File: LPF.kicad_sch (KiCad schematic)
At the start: 7 parts

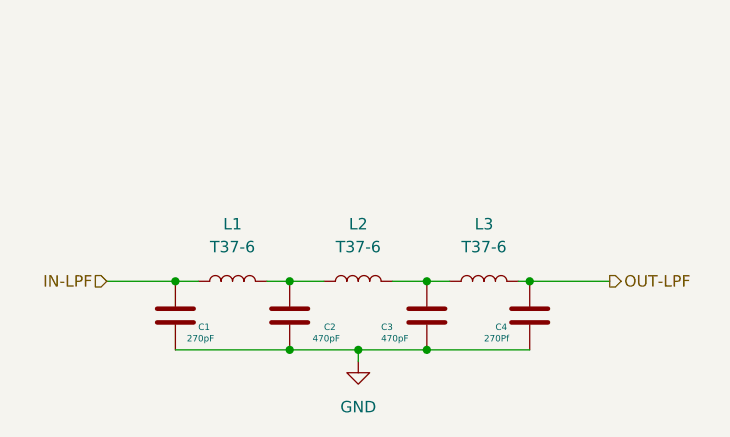
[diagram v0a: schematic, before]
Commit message: gg
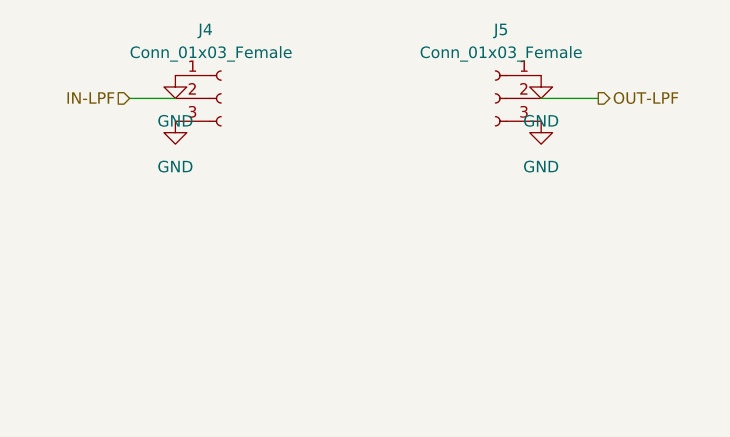
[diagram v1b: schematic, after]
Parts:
- removed C1: 270pF, Capacitor_SMD:C_1206_3216Metric, symbol Xenir:Capacitor
- removed C2, C3: 470pF, Capacitor_SMD:C_1206_3216Metric, symbol Xenir:Capacitor
- removed C4: 270Pf, Capacitor_SMD:C_1206_3216Metric, symbol Xenir:Capacitor
- removed L1, L2, L3: T37-6, Xenir:T37_Inductor, symbol Xenir:Inductor
- added J4, J5: Conn_01x03_Female, Connector_PinSocket_2.54mm:PinSocket_1x03_P2.54mm_Vertical, symbol Connector:Conn_01x03_Female
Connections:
- net GND: now also J4.1 (Pin_1), J4.3 (Pin_3), J5.1 (Pin_1), J5.3 (Pin_3)
- net IN-LPF: now also J4.2 (Pin_2)
- net OUT-LPF: now also J5.2 (Pin_2)
